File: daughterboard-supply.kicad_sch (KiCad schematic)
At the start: 19 parts, among them J9 39281103, SW1 1X03, U15 AP62301WU-7, U4 AP62301WU-7

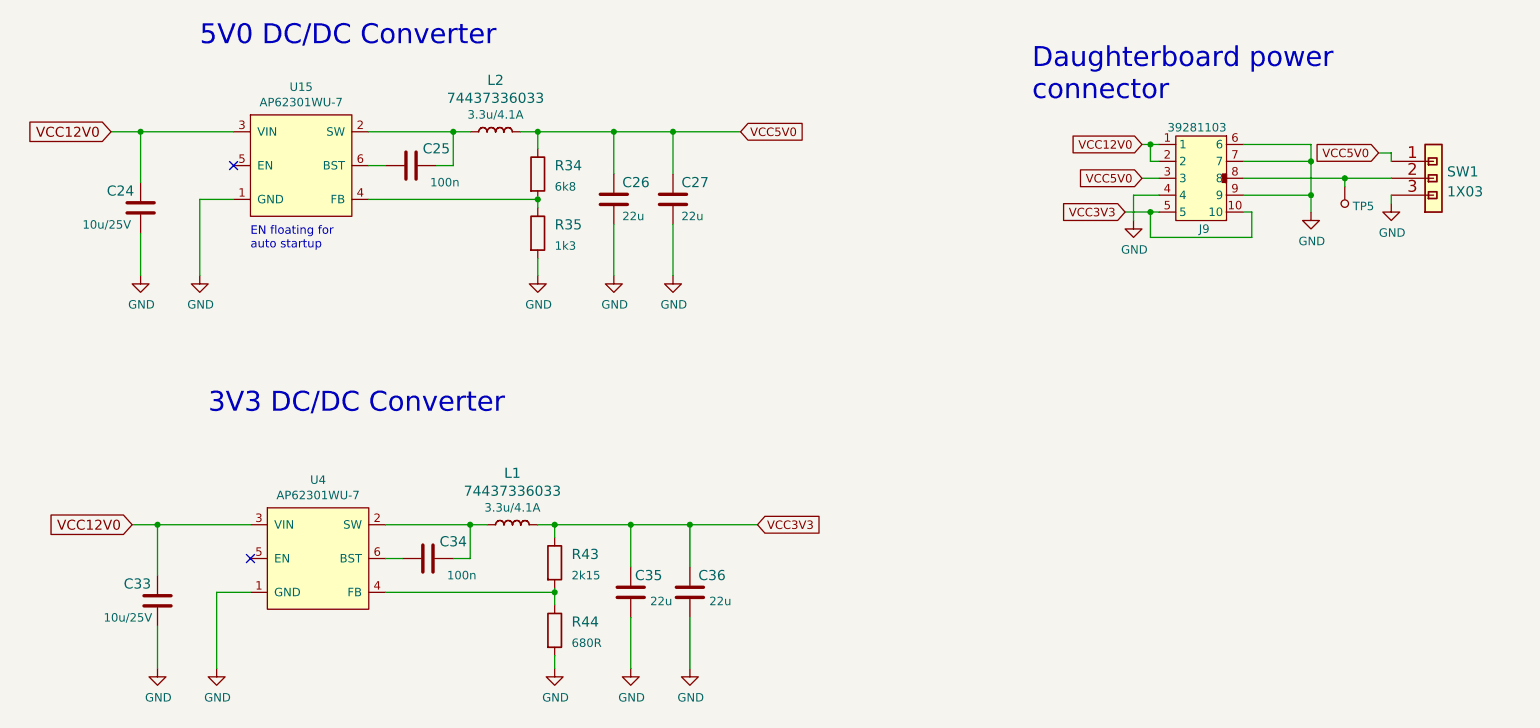
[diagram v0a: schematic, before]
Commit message: [#63472] Add OHP assets
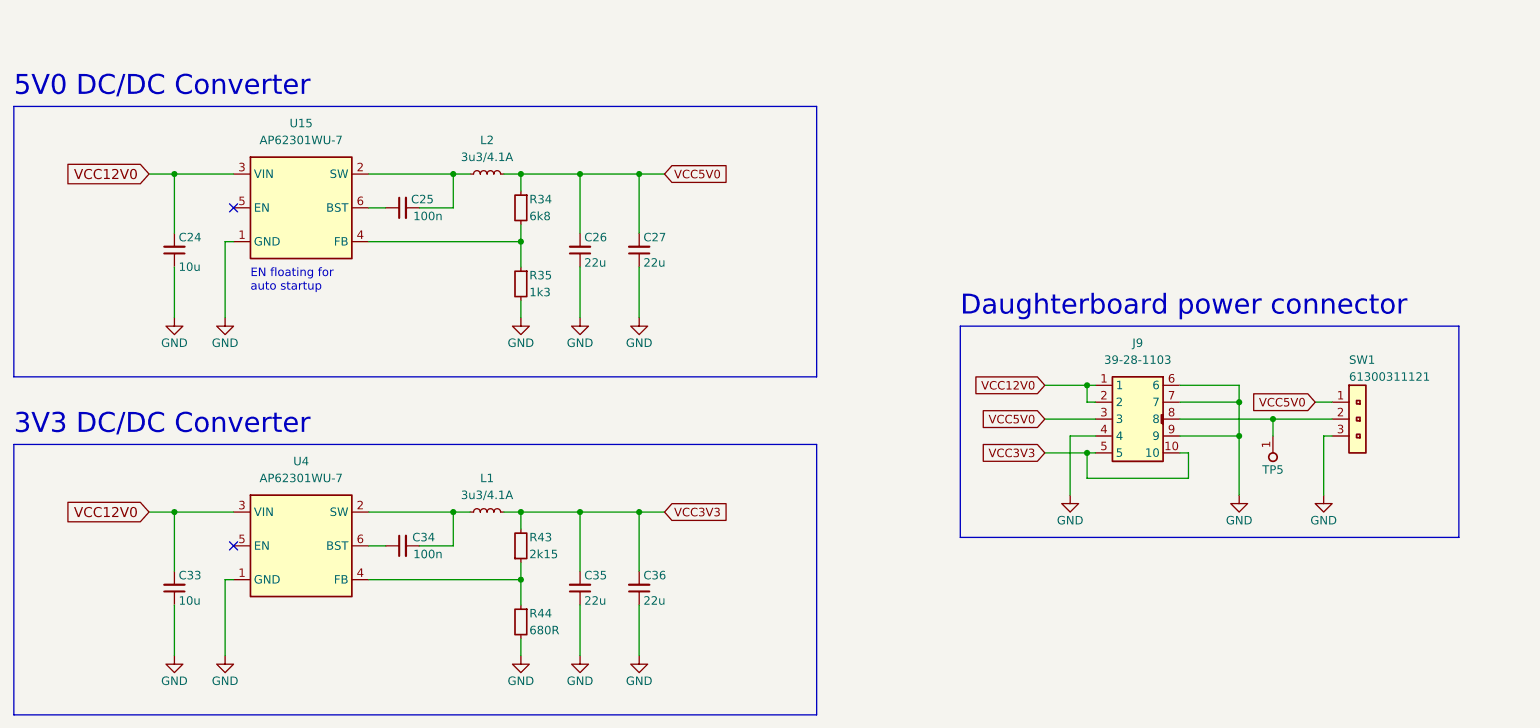
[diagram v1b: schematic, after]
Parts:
- removed J9: 39281103, d1600e-psu-breakout-board-footprints:MOLEX_39281103, symbol d1600e-psu-breakout-board:39281103
- removed TP5: TP_SMD1MM, antmicro-footprints:Testpoint_smd_1mm, symbol antmicroTestPoints:TP_SMD1MM
- added J9: Molex_Mini-Fit-Jr_2x5_39-28-1103, antmicro-footprints:MOLEX_39281103, symbol antmicroWire2BoardConnectors:Molex_Mini-Fit-Jr_2x5_39-28-1103
- added TP5: TP_1mm_SMD, antmicro-footprints:TP_SMD_1mm, symbol antmicroTestPoints:TP_1mm_SMD
- C24, C33: value C_10u_16V_0603 -> C_10u_25V_0603; footprint d1600e-psu-breakout-board-footprints:0603-cap -> antmicro-footprints:C_0603_1608Metric; symbol d1600e-psu-breakout-board:C_10u_25V_0603 -> antmicroCapacitors0603:C_10u_25V_0603; Author (none) -> Antmicro; License (none) -> Apache-2.0; Val 10u/25V -> 10u; Voltage (none) -> 25V
- C25, C34: footprint d1600e-psu-breakout-board-footprints:0402-cap -> antmicro-footprints:C_0402_1005Metric; symbol d1600e-psu-breakout-board:C_100n_0402 -> antmicroCapacitors0402:C_100n_0402; Author (none) -> Antmicro; Dielectric (none) -> X5R; License (none) -> Apache-2.0; Voltage (none) -> 50V
- C26, C27, C35, C36: footprint d1600e-psu-breakout-board-footprints:0603-cap -> antmicro-footprints:C_0603_1608Metric; symbol d1600e-psu-breakout-board:C_22u_0603 -> antmicroCapacitors0603:C_22u_0603; Author (none) -> Antmicro; License (none) -> Apache-2.0; Manufacturer MURATA -> Murata
- L1, L2: value 74437336033 -> L_3u3_4.1A_WE-LHMI-5030; footprint d1600e-psu-breakout-board-footprints:WE_74437336033 -> antmicro-footprints:L_WE-LHMI-5030; symbol d1600e-psu-breakout-board:74437336033 -> antmicroFixedInductors:L_3u3_4.1A_WE-LHMI-5030; Author (none) -> Antmicro; IMax (none) -> 4.1A; ISat (none) -> 5.45A; License (none) -> Apache-2.0; Manufacturer Wurth Elektronik -> Würth Elektronik; MaxCur 4.1A -> (none); Val 3.3u/4.1A -> 3u3/4.1A
- R34: footprint antmicro-footprints:0402-res -> antmicro-footprints:R_0402_1005Metric; Author (none) -> Antmicro; License (none) -> Apache-2.0; MPN RC0402FR-076K8L -> CR0402-FX-6801GLF; Manufacturer YAGEO_(PHYCOMP) -> Bourns; Tolerance (none) -> 1%
- R35: footprint antmicro-footprints:0402-res -> antmicro-footprints:R_0402_1005Metric; Author (none) -> Antmicro; License (none) -> Apache-2.0; MPN CR0402-FX-1301GLF -> CR0402-FX-1301GLF; Tolerance (none) -> 1%
- R43: footprint antmicro-footprints:0402-res -> antmicro-footprints:R_0402_1005Metric; Author (none) -> Antmicro; License (none) -> Apache-2.0; MPN CRCW04022K00FKED -> CR0402-FX-2151GLF; Manufacturer VISHAY -> Bourns; Tolerance (none) -> 1%
- R44: footprint antmicro-footprints:0402-res -> antmicro-footprints:R_0402_1005Metric; Author (none) -> Antmicro; License (none) -> Apache-2.0; MPN 0402WGJ0681TCE -> CR0402-FX-6800GLF; Manufacturer ROYAL_OHM -> Bourns; Tolerance (none) -> 1%
- SW1: value 1X03 -> PinHeader_1x3_P2.54mm_Drill1.1mm; footprint antmicro-footprints:MH_1X03_2.54 -> antmicro-footprints:PinHeader_1x3_P2.54mm_Drill1.1mm; symbol antmicroRectangularConnectorsHeadersMalePins:1X03 -> antmicroGenericPinHeaders:PinHeader_1x3_P2.54mm_Drill1.1mm; Author (none) -> Antmicro; License (none) -> Apache-2.0; Manufacturer Wurth Elektronik -> Würth Elektronik
- U15, U4: value AP62301WU-7 -> AP62301_TSOT; footprint d1600e-psu-breakout-board-footprints:TSOT23-6 -> antmicro-footprints:TSOT23-6; symbol d1600e-psu-breakout-board:AP62301WU-7 -> antmicroDCDCConverters:AP62301_TSOT; Author (none) -> Antmicro; License (none) -> Apache-2.0
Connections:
- net GND: now also C24.1, C26.1, C27.1, C33.1, C35.1, C36.1, J9.4, J9.6, J9.7, J9.9; no longer C24.2, C26.2, C27.2, C33.2, C35.2, C36.2
- net VCC12V0: now also C24.2, C33.2, J9.1, J9.2; no longer C24.1, C33.1
- net VCC3V3: now also C35.2, C36.2, R43.2, J9.10, J9.5; no longer C35.1, C36.1, R43.1
- net VCC5V0: now also C26.2, C27.2, J9.3; no longer C26.1, C27.1
- net at L2.1, U15.2 (SW): now also C25.2; no longer C25.1
- net at U15.6 (BST): now also C25.1; no longer C25.2
- net at L1.1, U4.2 (SW): now also C34.2; no longer C34.1
- net at R44.1, U4.4 (FB): now also R43.1; no longer R43.2
- net at U4.6 (BST): now also C34.1; no longer C34.2
- net at SW1.2: now also J9.8, TP5.1
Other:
- moved on the sheet: C24, C25, C26, C27, C33, C34, C35, C36, R34, R35, R43, R44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
